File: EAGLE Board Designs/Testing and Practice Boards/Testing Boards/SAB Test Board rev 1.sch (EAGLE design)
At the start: 105 parts, among them J1 CONNECTOR-4_μF_T_V_BLACK, J2 CONNECTOR-8_μF_T_V_BLACK, J3 CONNECTOR-4_μF_T_V_BLACK, J4 CONNECTOR-6_μF_T_V_BLACK, J6 CONNECTOR-4_μF_T_V_BLACK, U1 TPS54202DDCR, U10 MCP2515, U2 MCP2551, U6 OPAMP_1_CHANNEL_OPA991, U7 MAX3075, U8 LTC1563, U9 OPAMP_2_CHANNEL_OPA_2991, X1 CRYSTAL_16MHZ

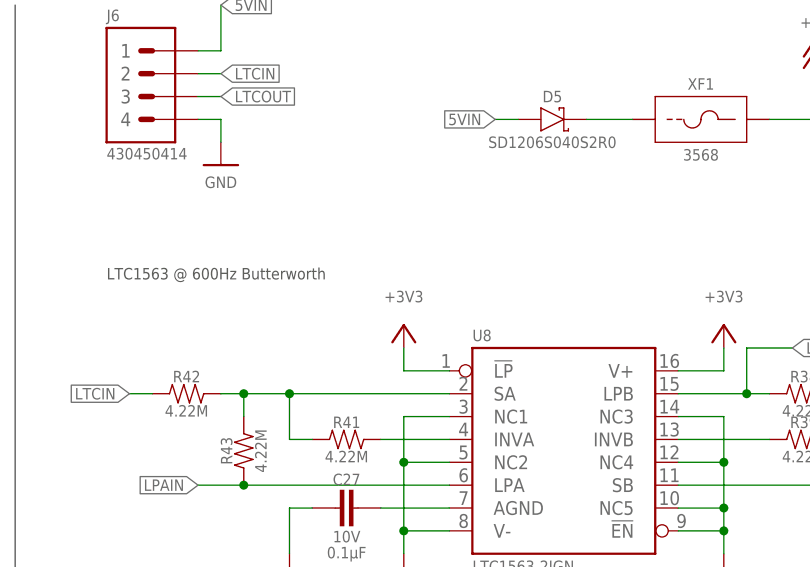
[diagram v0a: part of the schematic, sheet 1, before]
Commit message: Board changes
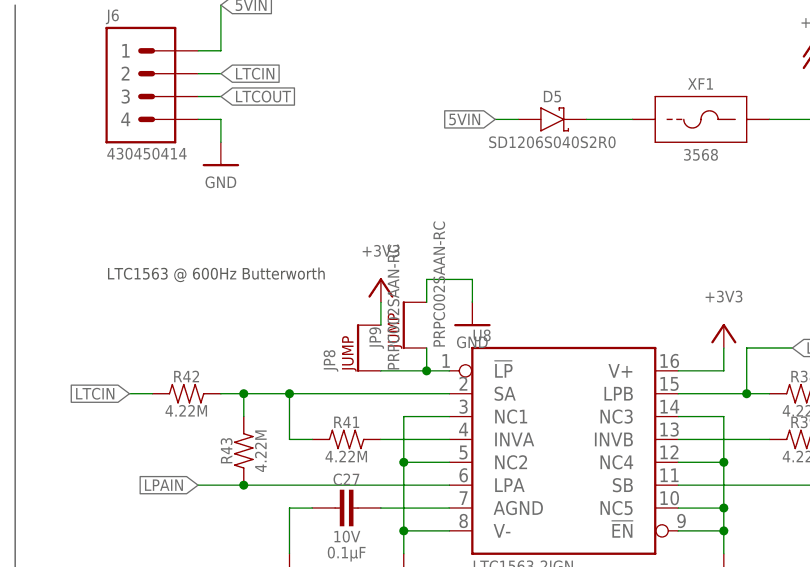
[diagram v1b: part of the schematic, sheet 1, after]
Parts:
- added JP8, JP9: JUMPER__1X02, HyTechDevices:JUMPER__1X02
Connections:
- new net N$10: JP8.1, JP9.1, U8.!LP
- net +3V3: now also JP8.2; no longer U8.!LP
- net GND: now also JP9.2
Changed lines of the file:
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@@
 <part name="R4" library="HyTechDevices" deviceset="RESISTOR_?_*" device="0603" technology="3.32K"/>
 <part name="D5" library="HyTechDevices" deviceset="SCHOTTKY_?_*" device="1206" technology="40V"/>
+<part name="JP8" library="HyTechDevices" deviceset="JUMPER_?_*" device="" technology="1X02"/>
+<part name="JP9" library="HyTechDevices" deviceset="JUMPER_?_*" device="" technology="1X02"/>
+<part name="P62" library="HyTechSupplies" deviceset="GND" device=""/>
 </parts>
 <sheets>
@@
 <attribute name="RESISTANCE" x="179.07" y="158.75" size="1.27" layer="96" rot="R90" align="top-center"/>
 </instance>
-<instance part="P59" gate="G$1" x="195.58" y="172.72" smashed="yes">
-<attribute name="VALUE" x="195.58" y="175.26" size="1.27" layer="96" align="bottom-center"/>
+<instance part="P59" gate="G$1" x="193.04" y="177.8" smashed="yes">
+<attribute name="VALUE" x="193.04" y="180.34" size="1.27" layer="96" align="bottom-center"/>
 </instance>
 <instance part="U2" gate="G$1" x="33.02" y="121.92" smashed="yes">
@@
 <attribute name="NAME" x="212.09" y="197.485" size="1.27" layer="95" align="bottom-center"/>
 <attribute name="MPN" x="212.09" y="193.675" size="1.27" layer="96" align="top-center"/>
+</instance>
+<instance part="JP8" gate="G$1" x="190.5" y="167.64" smashed="yes" rot="R90">
+<attribute name="NAME" x="187.96" y="167.64" size="1.27" layer="95" rot="R90"/>
+<attribute name="MPN" x="193.802" y="167.64" size="1.27" layer="96" rot="R90" align="top-left"/>
+</instance>
+<instance part="JP9" gate="G$1" x="195.58" y="170.18" smashed="yes" rot="R90">
+<attribute name="NAME" x="193.04" y="170.18" size="1.27" layer="95" rot="R90"/>
+<attribute name="MPN" x="198.882" y="170.18" size="1.27" layer="96" rot="R90" align="top-left"/>
+</instance>
+<instance part="P62" gate="1" x="203.2" y="172.72" smashed="yes">
+<attribute name="VALUE" x="203.2" y="171.45" size="1.27" layer="96" align="top-center"/>
 </instance>
 </instances>
@@
 <junction x="129.54" y="154.94"/>
 </segment>
+<segment>
+<pinref part="JP9" gate="G$1" pin="2"/>
+<wire x1="198.12" y1="175.26" x2="198.12" y2="177.8" width="0.1524" layer="91"/>
+<wire x1="198.12" y1="177.8" x2="203.2" y2="177.8" width="0.1524" layer="91"/>
+<wire x1="203.2" y1="177.8" x2="203.2" y2="175.26" width="0.1524" layer="91"/>
+<pinref part="P62" gate="1" pin="GND"/>
+</segment>
 </net>
 <net name="TXCAN" class="0">
@@
 <pinref part="U8" gate="G$1" pin="V+"/>
 <wire x1="231.14" y1="167.64" x2="226.06" y2="167.64" width="0.1524" layer="91"/>
-</segment>
-<segment>
-<pinref part="P59" gate="G$1" pin="+3V3"/>
-<pinref part="U8" gate="G$1" pin="!LP"/>
-<wire x1="195.58" y1="170.18" x2="195.58" y2="167.64" width="0.1524" layer="91"/>
-<wire x1="195.58" y1="167.64" x2="200.66" y2="167.64" width="0.1524" layer="91"/>
 </segment>
 <segment>
@@
 <wire x1="129.54" y1="167.64" x2="139.7" y2="167.64" width="0.1524" layer="91"/>
 <wire x1="139.7" y1="167.64" x2="139.7" y2="162.56" width="0.1524" layer="91"/>
+</segment>
+<segment>
+<pinref part="JP8" gate="G$1" pin="2"/>
+<pinref part="P59" gate="G$1" pin="+3V3"/>
+<wire x1="193.04" y1="172.72" x2="193.04" y2="175.26" width="0.1524" layer="91"/>
 </segment>
 </net>
@@
 </segment>
 </net>
+<net name="N$10" class="0">
+<segment>
+<pinref part="U8" gate="G$1" pin="!LP"/>
+<wire x1="193.04" y1="167.64" x2="198.12" y2="167.64" width="0.1524" layer="91"/>
+<pinref part="JP8" gate="G$1" pin="1"/>
+<wire x1="198.12" y1="167.64" x2="200.66" y2="167.64" width="0.1524" layer="91"/>
+<wire x1="198.12" y1="167.64" x2="198.12" y2="170.18" width="0.1524" layer="91"/>
+<junction x="198.12" y="167.64"/>
+<pinref part="JP9" gate="G$1" pin="1"/>
+</segment>
+</net>
